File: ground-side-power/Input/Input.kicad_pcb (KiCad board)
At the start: 2 copper layers, 95.8 x 122.1 mm, 41 parts, among them J1 Battery Terminals, J2 Battery Terminals, J26 Conn_01x02_Female, J3 Battery Terminals, J4 Battery Terminals, J5 874270842, J6 874270842, J7 ATX-24, J8 Conn_01x03_Female, J9 Conn_01x03_Female, K1 AZ2150-1A-12DEF, M1 Fan_PC_Chassis, SW1 GRB234A2NABA1, U1 INA180, U2 INA180

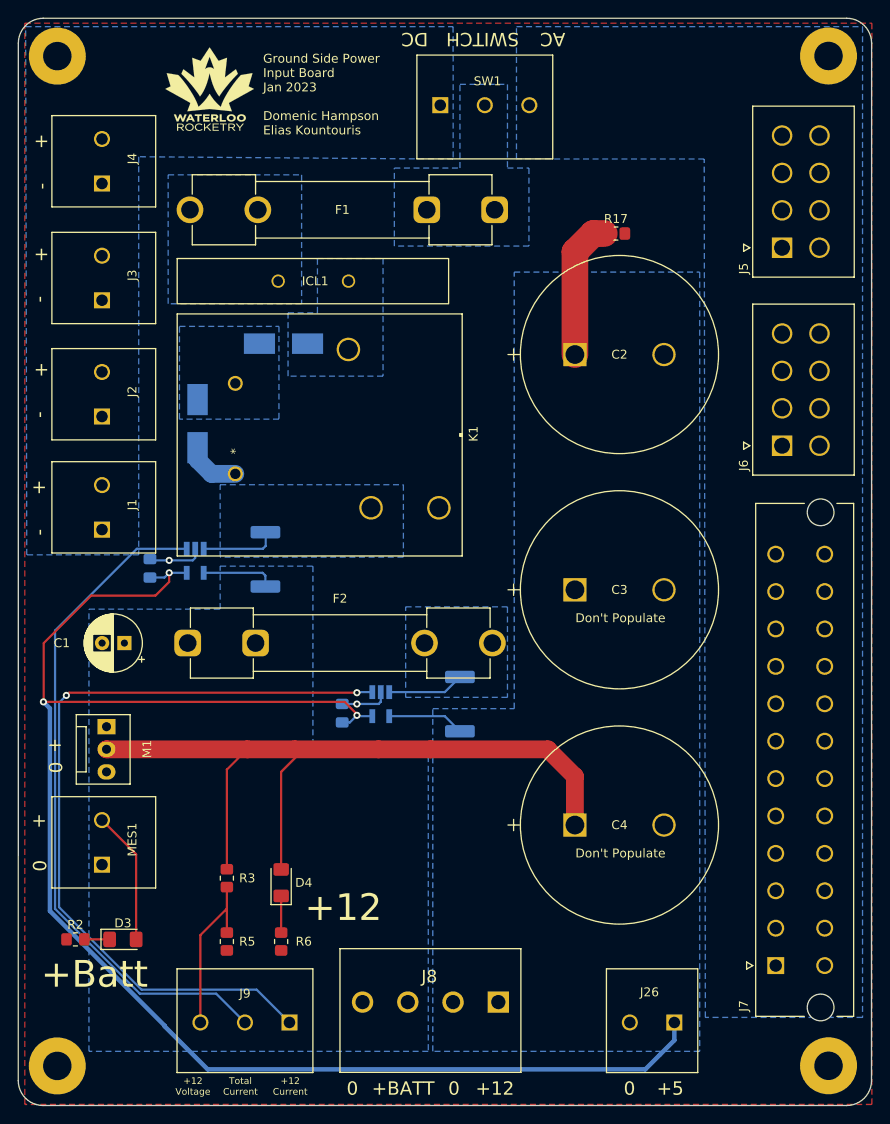
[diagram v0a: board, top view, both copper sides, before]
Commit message: Added Gerbers
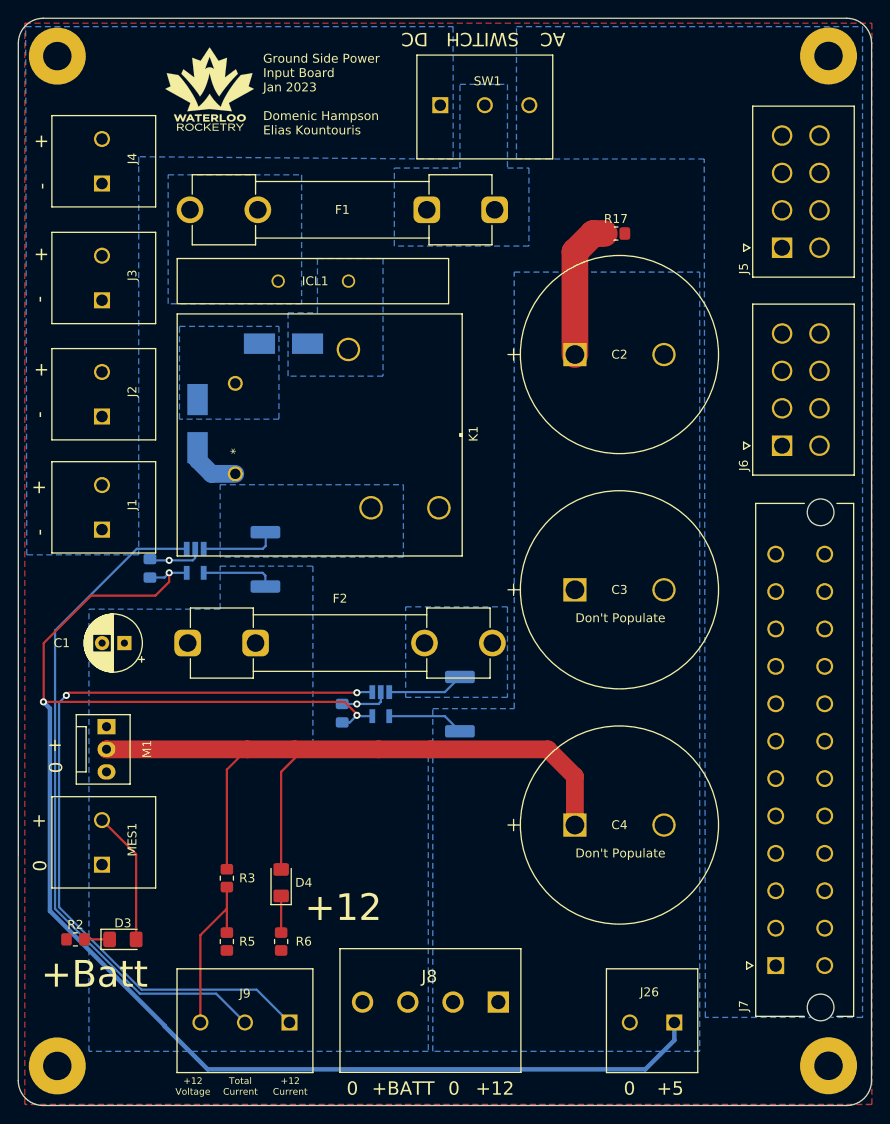
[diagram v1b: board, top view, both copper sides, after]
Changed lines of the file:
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@@
       (layerselection 0x00010fc_ffffffff)
       (disableapertmacros false)
-      (usegerberextensions false)
-      (usegerberattributes true)
-      (usegerberadvancedattributes true)
-      (creategerberjobfile true)
+      (usegerberextensions true)
+      (usegerberattributes false)
+      (usegerberadvancedattributes false)
+      (creategerberjobfile false)
       (svguseinch false)
       (svgprecision 6)
@@
       (psa4output false)
       (plotreference true)
-      (plotvalue true)
+      (plotvalue false)
       (plotinvisibletext false)
       (sketchpadsonfab false)
-      (subtractmaskfromsilk false)
+      (subtractmaskfromsilk true)
       (outputformat 1)
       (mirror false)
-      (drillshape 1)
+      (drillshape 0)
       (scaleselection 1)
-      (outputdirectory "")
+      (outputdirectory "../Gerbers/Input/")
     )
   )
@@
     (fp_line (start -1.2 -0.8) (end -1.6 -0.4) (layer "F.Fab") (width 0.1))
     (fp_line (start -1.6 -0.4) (end -1.6 0.8) (layer "F.Fab") (width 0.1))
-    (pad "1" smd roundrect (at -1.4875 0) (size 1.425 1.75) (layers "F.Cu" "F.Paste" "F.Mask") (roundrect_rratio 0.175439)
+    (pad "1" smd roundrect (at -1.4875 0) (size 1.425 1.75) (layers "F.Cu" "F.Paste" "F.Mask") (roundrect_rratio 0.1754392982)
       (net 7 "Net-(D3-Pad1)") (pinfunction "K") (pintype "passive"))
-    (pad "2" smd roundrect (at 1.4875 0) (size 1.425 1.75) (layers "F.Cu" "F.Paste" "F.Mask") (roundrect_rratio 0.175439)
+    (pad "2" smd roundrect (at 1.4875 0) (size 1.425 1.75) (layers "F.Cu" "F.Paste" "F.Mask") (roundrect_rratio 0.1754392982)
       (net 1 "+BATT") (pinfunction "A") (pintype "passive"))
     (model "${KICAD6_3DMODEL_DIR}/Diode_SMD.3dshapes/D_1206_3216Metric.wrl"
@@
     (fp_line (start 1 0.625) (end -1 0.625) (layer "F.Fab") (width 0.1))
     (fp_line (start -1 -0.625) (end 1 -0.625) (layer "F.Fab") (width 0.1))
-    (pad "1" smd roundrect (at -1 0 90) (size 1.2 1.4) (layers "F.Cu" "F.Paste" "F.Mask") (roundrect_rratio 0.208333)
+    (pad "1" smd roundrect (at -1 0 90) (size 1.2 1.4) (layers "F.Cu" "F.Paste" "F.Mask") (roundrect_rratio 0.2083333333)
       (net 2 "GND") (pintype "passive"))
-    (pad "2" smd roundrect (at 1 0 90) (size 1.2 1.4) (layers "F.Cu" "F.Paste" "F.Mask") (roundrect_rratio 0.208333)
+    (pad "2" smd roundrect (at 1 0 90) (size 1.2 1.4) (layers "F.Cu" "F.Paste" "F.Mask") (roundrect_rratio 0.2083333333)
       (net 8 "Net-(D4-Pad1)") (pintype "passive"))
     (model "${KICAD6_3DMODEL_DIR}/Resistor_SMD.3dshapes/R_0805_2012Metric.wrl"
@@
     (fp_line (start -1 0.625) (end -1 -0.625) (layer "F.Fab") (width 0.1))
     (fp_line (start 1 0.625) (end -1 0.625) (layer "F.Fab") (width 0.1))
-    (pad "1" smd roundrect (at -1 0 270) (size 1.2 1.4) (layers "F.Cu" "F.Paste" "F.Mask") (roundrect_rratio 0.208333)
+    (pad "1" smd roundrect (at -1 0 270) (size 1.2 1.4) (layers "F.Cu" "F.Paste" "F.Mask") (roundrect_rratio 0.2083333333)
       (net 3 "+12V") (pintype "passive"))
-    (pad "2" smd roundrect (at 1 0 270) (size 1.2 1.4) (layers "F.Cu" "F.Paste" "F.Mask") (roundrect_rratio 0.208333)
+    (pad "2" smd roundrect (at 1 0 270) (size 1.2 1.4) (layers "F.Cu" "F.Paste" "F.Mask") (roundrect_rratio 0.2083333333)
       (net 22 "/12_VOLTAGE") (pintype "passive"))
     (model "${KICAD6_3DMODEL_DIR}/Resistor_SMD.3dshapes/R_0805_2012Metric.wrl"
@@
     (fp_line (start 1.6 0.8) (end 1.6 -0.8) (layer "F.Fab") (width 0.1))
     (fp_line (start -1.2 -0.8) (end -1.6 -0.4) (layer "F.Fab") (width 0.1))
-    (pad "1" smd roundrect (at -1.4875 0 90) (size 1.425 1.75) (layers "F.Cu" "F.Paste" "F.Mask") (roundrect_rratio 0.175439)
+    (pad "1" smd roundrect (at -1.4875 0 90) (size 1.425 1.75) (layers "F.Cu" "F.Paste" "F.Mask") (roundrect_rratio 0.1754392982)
       (net 8 "Net-(D4-Pad1)") (pinfunction "K") (pintype "passive"))
-    (pad "2" smd roundrect (at 1.4875 0 90) (size 1.425 1.75) (layers "F.Cu" "F.Paste" "F.Mask") (roundrect_rratio 0.175439)
+    (pad "2" smd roundrect (at 1.4875 0 90) (size 1.425 1.75) (layers "F.Cu" "F.Paste" "F.Mask") (roundrect_rratio 0.1754392982)
       (net 3 "+12V") (pinfunction "A") (pintype "passive"))
     (model "${KICAD6_3DMODEL_DIR}/Diode_SMD.3dshapes/D_1206_3216Metric.wrl"
@@
     (fp_line (start -1 0.625) (end -1 -0.625) (layer "F.Fab") (width 0.1))
     (fp_line (start 1 -0.625) (end 1 0.625) (layer "F.Fab") (width 0.1))
-    (pad "1" smd roundrect (at -1 0) (size 1.2 1.4) (layers "F.Cu" "F.Paste" "F.Mask") (roundrect_rratio 0.208333)
+    (pad "1" smd roundrect (at -1 0) (size 1.2 1.4) (layers "F.Cu" "F.Paste" "F.Mask") (roundrect_rratio 0.2083333333)
       (net 3 "+12V") (pintype "passive"))
-    (pad "2" smd roundrect (at 1 0) (size 1.2 1.4) (layers "F.Cu" "F.Paste" "F.Mask") (roundrect_rratio 0.208333)
+    (pad "2" smd roundrect (at 1 0) (size 1.2 1.4) (layers "F.Cu" "F.Paste" "F.Mask") (roundrect_rratio 0.2083333333)
       (net 2 "GND") (pintype "passive"))
     (model "${KICAD6_3DMODEL_DIR}/Resistor_SMD.3dshapes/R_0805_2012Metric.wrl"
@@
     (fp_line (start 1 0.625) (end -1 0.625) (layer "F.Fab") (width 0.1))
     (fp_line (start 1 -0.625) (end 1 0.625) (layer "F.Fab") (width 0.1))
-    (pad "1" smd roundrect (at -1 0 270) (size 1.2 1.4) (layers "F.Cu" "F.Paste" "F.Mask") (roundrect_rratio 0.208333)
+    (pad "1" smd roundrect (at -1 0 270) (size 1.2 1.4) (layers "F.Cu" "F.Paste" "F.Mask") (roundrect_rratio 0.2083333333)
       (net 22 "/12_VOLTAGE") (pintype "passive"))
-    (pad "2" smd roundrect (at 1 0 270) (size 1.2 1.4) (layers "F.Cu" "F.Paste" "F.Mask") (roundrect_rratio 0.208333)
+    (pad "2" smd roundrect (at 1 0 270) (size 1.2 1.4) (layers "F.Cu" "F.Paste" "F.Mask") (roundrect_rratio 0.2083333333)
       (net 2 "GND") (pintype "passive"))
     (model "${KICAD6_3DMODEL_DIR}/Resistor_SMD.3dshapes/R_0805_2012Metric.wrl"
@@
     (fp_line (start 1 -0.625) (end 1 0.625) (layer "F.Fab") (width 0.1))
     (fp_line (start 1 0.625) (end -1 0.625) (layer "F.Fab") (width 0.1))
-    (pad "1" smd roundrect (at -1 0) (size 1.2 1.4) (layers "F.Cu" "F.Paste" "F.Mask") (roundrect_rratio 0.208333)
+    (pad "1" smd roundrect (at -1 0) (size 1.2 1.4) (layers "F.Cu" "F.Paste" "F.Mask") (roundrect_rratio 0.2083333333)
       (net 2 "GND") (pintype "passive"))
-    (pad "2" smd roundrect (at 1 0) (size 1.2 1.4) (layers "F.Cu" "F.Paste" "F.Mask") (roundrect_rratio 0.208333)
+    (pad "2" smd roundrect (at 1 0) (size 1.2 1.4) (layers "F.Cu" "F.Paste" "F.Mask") (roundrect_rratio 0.2083333333)
       (net 7 "Net-(D3-Pad1)") (pintype "passive"))
     (model "${KICAD6_3DMODEL_DIR}/Resistor_SMD.3dshapes/R_0805_2012Metric.wrl"
@@
     (fp_line (start 1 0.625) (end 1 -0.625) (layer "B.Fab") (width 0.1))
     (fp_line (start 1 -0.625) (end -1 -0.625) (layer "B.Fab") (width 0.1))
-    (pad "1" smd roundrect (at -1.0375 0 270) (size 1.175 1.45) (layers "B.Cu" "B.Paste" "B.Mask") (roundrect_rratio 0.212766)
+    (pad "1" smd roundrect (at -1.0375 0 270) (size 1.175 1.45) (layers "B.Cu" "B.Paste" "B.Mask") (roundrect_rratio 0.2127659574)
       (net 2 "GND") (pintype "passive"))
-    (pad "2" smd roundrect (at 1.0375 0 270) (size 1.175 1.45) (layers "B.Cu" "B.Paste" "B.Mask") (roundrect_rratio 0.212766)
+    (pad "2" smd roundrect (at 1.0375 0 270) (size 1.175 1.45) (layers "B.Cu" "B.Paste" "B.Mask") (roundrect_rratio 0.2127659574)
       (net 4 "+5V") (pintype "passive"))
     (model "${KICAD6_3DMODEL_DIR}/Capacitor_SMD.3dshapes/C_0805_2012Metric.wrl"
@@
     (fp_line (start 1 0.625) (end 1 -0.625) (layer "B.Fab") (width 0.1))
     (fp_line (start -1 -0.625) (end -1 0.625) (layer "B.Fab") (width 0.1))
-    (pad "1" smd roundrect (at -1.0375 0 270) (size 1.175 1.45) (layers "B.Cu" "B.Paste" "B.Mask") (roundrect_rratio 0.212766)
+    (pad "1" smd roundrect (at -1.0375 0 270) (size 1.175 1.45) (layers "B.Cu" "B.Paste" "B.Mask") (roundrect_rratio 0.2127659574)
       (net 2 "GND") (pintype "passive"))
-    (pad "2" smd roundrect (at 1.0375 0 270) (size 1.175 1.45) (layers "B.Cu" "B.Paste" "B.Mask") (roundrect_rratio 0.212766)
+    (pad "2" smd roundrect (at 1.0375 0 270) (size 1.175 1.45) (layers "B.Cu" "B.Paste" "B.Mask") (roundrect_rratio 0.2127659574)
       (net 4 "+5V") (pintype "passive"))
     (model "${KICAD6_3DMODEL_DIR}/Capacitor_SMD.3dshapes/C_0805_2012Metric.wrl"
@@
     (fp_line (start -3.15 1.6) (end 3.15 1.6) (layer "B.Fab") (width 0.1))
     (fp_line (start 3.15 1.6) (end 3.15 -1.6) (layer "B.Fab") (width 0.1))
-    (pad "1" smd roundrect (at -3.05 0 270) (size 1.4 3.35) (layers "B.Cu" "B.Paste" "B.Mask") (roundrect_rratio 0.178571)
+    (pad "1" smd roundrect (at -3.05 0 270) (size 1.4 3.35) (layers "B.Cu" "B.Paste" "B.Mask") (roundrect_rratio 0.1785707143)
       (net 23 "/Sys_Sense+") (pintype "passive"))
-    (pad "2" smd roundrect (at 3.05 0 270) (size 1.4 3.35) (layers "B.Cu" "B.Paste" "B.Mask") (roundrect_rratio 0.178571)
+    (pad "2" smd roundrect (at 3.05 0 270) (size 1.4 3.35) (layers "B.Cu" "B.Paste" "B.Mask") (roundrect_rratio 0.1785707143)
       (net 1 "+BATT") (pintype "passive"))
     (model "${KICAD6_3DMODEL_DIR}/Resistor_SMD.3dshapes/R_2512_6332Metric.wrl"
@@
     (fp_line (start 3.15 1.6) (end 3.15 -1.6) (layer "B.Fab") (width 0.1))
     (fp_line (start -3.15 -1.6) (end -3.15 1.6) (layer "B.Fab") (width 0.1))
-    (pad "1" smd roundrect (at -3.05 0 270) (size 1.4 3.35) (layers "B.Cu" "B.Paste" "B.Mask") (roundrect_rratio 0.178571)
+    (pad "1" smd roundrect (at -3.05 0 270) (size 1.4 3.35) (layers "B.Cu" "B.Paste" "B.Mask") (roundrect_rratio 0.1785707143)
       (net 11 "/12V_Sense+") (pintype "passive"))
-    (pad "2" smd roundrect (at 3.05 0 270) (size 1.4 3.35) (layers "B.Cu" "B.Paste" "B.Mask") (roundrect_rratio 0.178571)
+    (pad "2" smd roundrect (at 3.05 0 270) (size 1.4 3.35) (layers "B.Cu" "B.Paste" "B.Mask") (roundrect_rratio 0.1785707143)
       (net 3 "+12V") (pintype "passive"))
     (model "${KICAD6_3DMODEL_DIR}/Resistor_SMD.3dshapes/R_2512_6332Metric.wrl"
